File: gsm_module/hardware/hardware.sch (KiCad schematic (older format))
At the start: 58 parts, among them J1 Screw_Terminal_01x04, J2 Conn_01x06_Female, J3 Conn_01x06_Female, J4 Programming interface, J5 SWD Debugging Interface, U1 XL1509-ADJ, U2 AMS1117-3.3, U2 XL1509-ADJ, U3 STM32F030F4Px, U4 MCP2515-xSO, U5 MCP2551-I-SN

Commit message: Rev 1 schematic all footprints done
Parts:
- removed JP1, JP2, JP? (x3): Jumper, symbol Device:Jumper
- removed JP3, JP4: Programming Jumpers, symbol Device:Jumper
- removed JP?: SPI Jumpers, symbol Device:Jumper
- removed U2: XL1509-ADJ, symbol xl1509:XL1509
- added C11, C5: 5nF, Capacitor_THT:C_Disc_D4.3mm_W1.9mm_P5.00mm, symbol Device:C
- added J10, J11, J12, J13, J6, J7, J8, J9: Conn_01x02_Male, Connector_PinHeader_1.00mm:PinHeader_1x02_P1.00mm_Vertical, symbol Connector:Conn_01x02_Male
- added U10: XL1509-ADJ, Package_SO:SOIC-8-1EP_3.9x4.9mm_P1.27mm_EP2.29x3mm, symbol xl1509:XL1509
- C1, C2: footprint (none) -> Capacitor_THT:C_Disc_D4.3mm_W1.9mm_P5.00mm
- C10: renamed from C9; footprint (none) -> Capacitor_THT:C_Disc_D4.3mm_W1.9mm_P5.00mm
- C12, C13: renamed from C?; footprint (none) -> Capacitor_THT:C_Disc_D4.3mm_W1.9mm_P5.00mm
- C3, C4, polcap1, polcap3, polcap4: footprint (none) -> Capacitor_THT:CP_Radial_D8.0mm_P3.50mm
- C6: renamed from C5; footprint (none) -> Capacitor_THT:C_Disc_D4.3mm_W1.9mm_P5.00mm
- C7: renamed from C6; footprint (none) -> Capacitor_THT:C_Disc_D4.3mm_W1.9mm_P5.00mm
- C8: renamed from C7; footprint (none) -> Capacitor_THT:C_Disc_D4.3mm_W1.9mm_P5.00mm
- C9: renamed from C8; footprint (none) -> Capacitor_THT:C_Disc_D4.3mm_W1.9mm_P5.00mm
- D1, D2: value 1N5820 -> MBR360
- D3, D4, D5: footprint (none) -> LED_THT:LED_D5.0mm
- J1: footprint (none) -> Connector_PinHeader_1.27mm:PinHeader_1x04_P1.27mm_Vertical
- J2: value Conn_01x06_Female -> SIM800C Module; footprint (none) -> Connector_PinHeader_1.27mm:PinHeader_1x06_P1.27mm_Vertical
- J3: value Conn_01x06_Female -> SIM800C Module Side A; footprint (none) -> Connector_PinHeader_1.27mm:PinHeader_1x06_P1.27mm_Vertical
- J4: footprint (none) -> Connector_PinHeader_1.00mm:PinHeader_1x05_P1.00mm_Vertical
- J5: footprint (none) -> Connector_PinHeader_1.00mm:PinHeader_1x02_P1.00mm_Vertical
- L1, L2: footprint (none) -> Resistor_THT:R_Axial_DIN0207_L6.3mm_D2.5mm_P10.16mm_Horizontal
- R1, R10, R11, R2, R3, R4, R5, R6, R7, R8, R9: footprint (none) -> Resistor_THT:R_Axial_DIN0309_L9.0mm_D3.2mm_P12.70mm_Horizontal
- R12: renamed from R13; footprint (none) -> Resistor_THT:R_Axial_DIN0309_L9.0mm_D3.2mm_P12.70mm_Horizontal
- R13: renamed from R14; footprint (none) -> Resistor_THT:R_Axial_DIN0309_L9.0mm_D3.2mm_P12.70mm_Horizontal
- R14: renamed from R12; footprint (none) -> Resistor_THT:R_Axial_DIN0309_L9.0mm_D3.2mm_P12.70mm_Horizontal
- R15, R16: renamed from R?; footprint (none) -> Resistor_THT:R_Axial_DIN0309_L9.0mm_D3.2mm_P12.70mm_Horizontal
- U1: footprint (none) -> Package_SO:SOIC-8-1EP_3.9x4.9mm_P1.27mm_EP2.29x3mm
- Y1: renamed from Y?; footprint (none) -> Crystal:Crystal_HC18-U_Vertical
- renumbered U4 to U3, U3 to U4
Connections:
- wire segments 136 -> 151

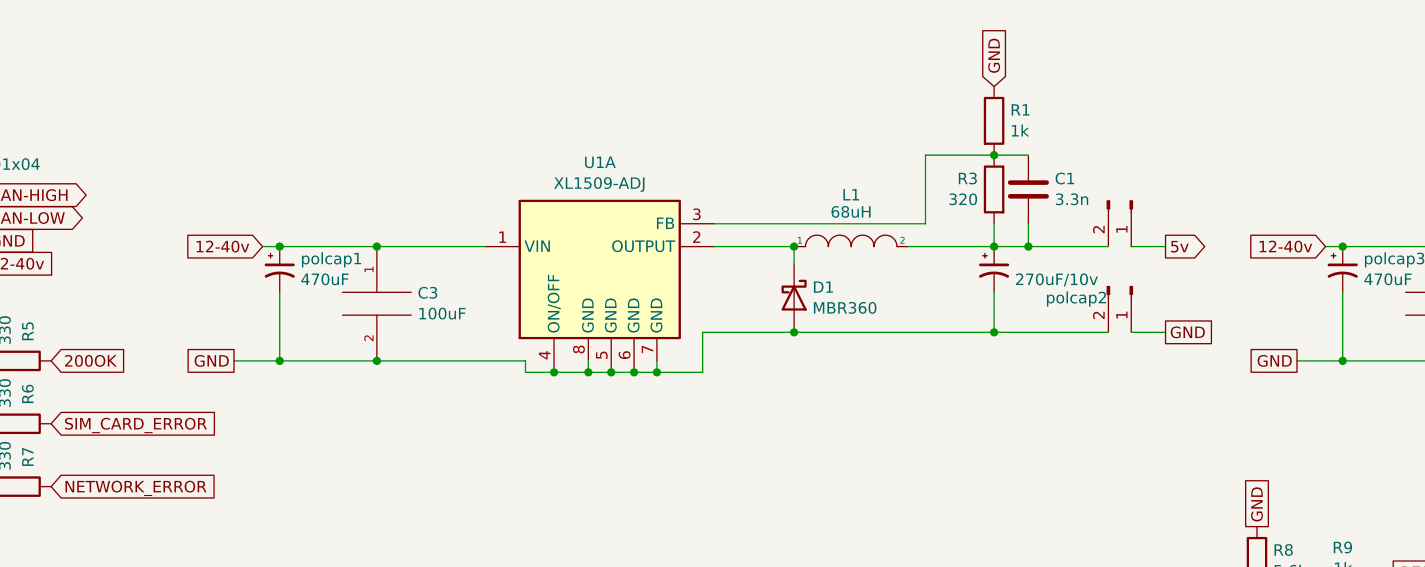
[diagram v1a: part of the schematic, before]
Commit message: rev 1.5 final
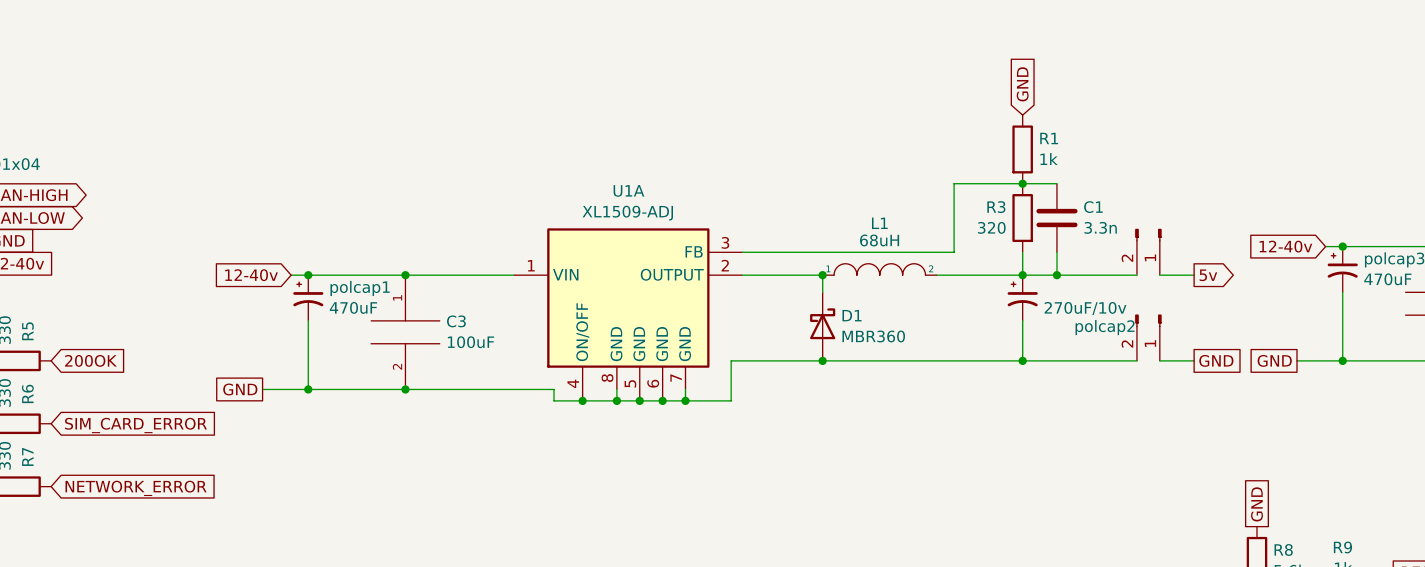
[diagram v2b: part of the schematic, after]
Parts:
- polcap2: footprint (none) -> Capacitor_THT:CP_Radial_D8.0mm_P3.50mm
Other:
- moved on the sheet: C1, C3, D1, L1, R1, R3, U1A, polcap1, polcap2
